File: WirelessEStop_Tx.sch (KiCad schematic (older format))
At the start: 75 parts, among them IC1 DRV2605LDGSR, J1 U.FL-R-SMT(01), J2 Conn_01x02, J3 USB_B_Micro, J4 Conn_01x02, Q1 Q_NMOS_GSD, SW1 SW_DIP_x01, SW2 SW_DIP_x01, SW3 SW_Push, SW4 SW_Push, SW5 SW_DIP_x01, SW6 SW_SPDT, U1 ESP8266EX, U2 25Q128FV, U3 CH340, U4 MCP73831T-2ACI_OT, U5 TPS73633DBVR, Y1 Crystal_GND24

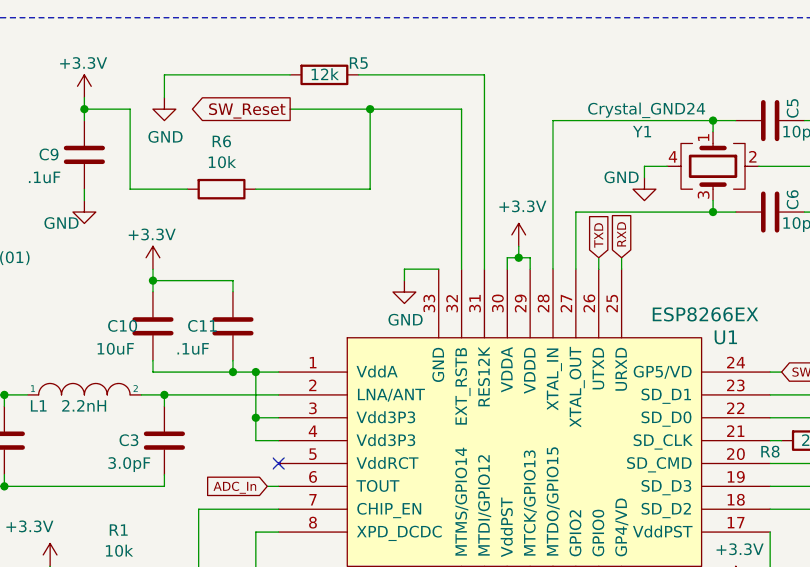
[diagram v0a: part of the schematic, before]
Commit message: Eli suck my dick
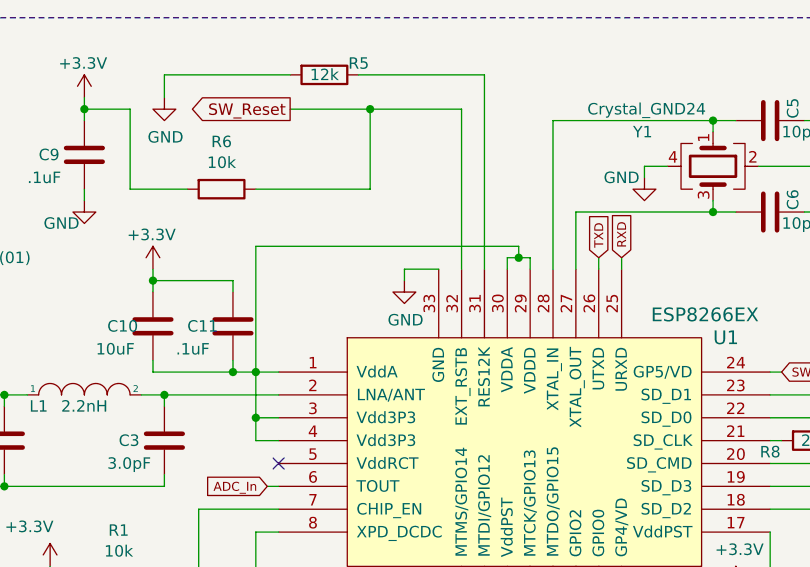
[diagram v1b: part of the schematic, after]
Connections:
- net +3V3: no longer U1.29 (VDDD), U1.30 (VDDA)
- net at C10.2, C11.2, U1.1 (VddA)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: now also U1.29 (VDDD), U1.30 (VDDA)
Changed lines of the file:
@@
-$EndComp
-$Comp
-L power:+3.3V #PWR013
-U 1 1 5DE96AF6
-P 3550 1850
-F 0 "#PWR013" H 3550 1700 50  0001 C CNN
-F 1 "+3.3V" H 3565 2023 50  0000 C CNN
-F 2 "" H 3550 1850 50  0001 C CNN
-F 3 "" H 3550 1850 50  0001 C CNN
-	1    3550 1850
-	1    0    0    -1
 $EndComp
 $Comp
@@
 Text Notes 7750 5900 1    30   ~ 0
 Pink LED
+Wire Wire Line
+	3550 1850 2400 1850
+Wire Wire Line
+	2400 1850 2400 2400
 $EndSCHEMATC
